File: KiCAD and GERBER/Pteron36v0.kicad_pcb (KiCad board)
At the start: 2 copper layers, 140.1 x 108.1 mm, 56 parts, among them J1 AudioJack4, J2 AudioJack4, J3 Conn_01x04, SW10 SW_PUSH, SW12 SW_PUSH, SW13 SW_PUSH, SW14 SW_PUSH, SW15 SW_PUSH, SW17 SW_PUSH, SW18 SW_PUSH, SW19 SW_PUSH, SW20 SW_PUSH, SW22 SW_PUSH, SW23 SW_PUSH, SW24 SW_PUSH, SW26 SW_PUSH, SW27 SW_PUSH, SW28 SW_PUSH, SW7 SW_PUSH, SW8 SW_PUSH, SW9 SW_PUSH, U1 ProMicro

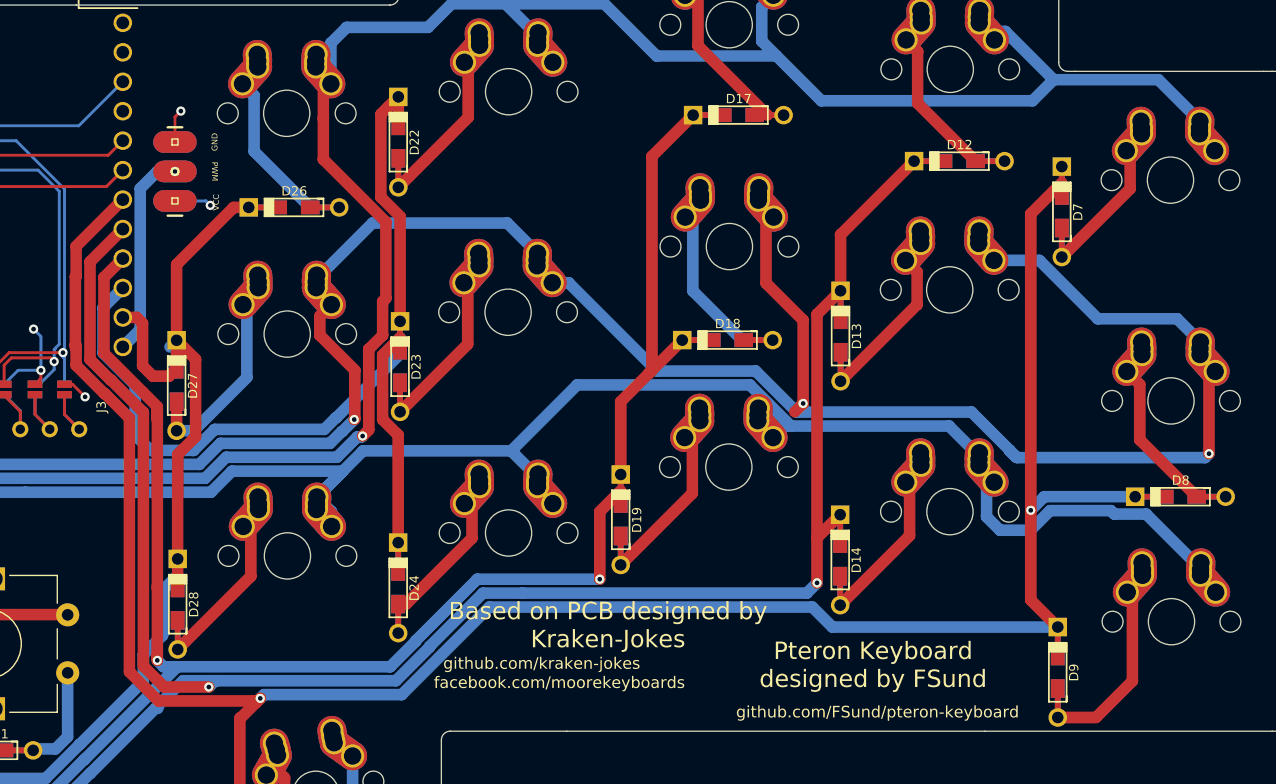
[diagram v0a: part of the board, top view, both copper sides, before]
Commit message: updated pcb
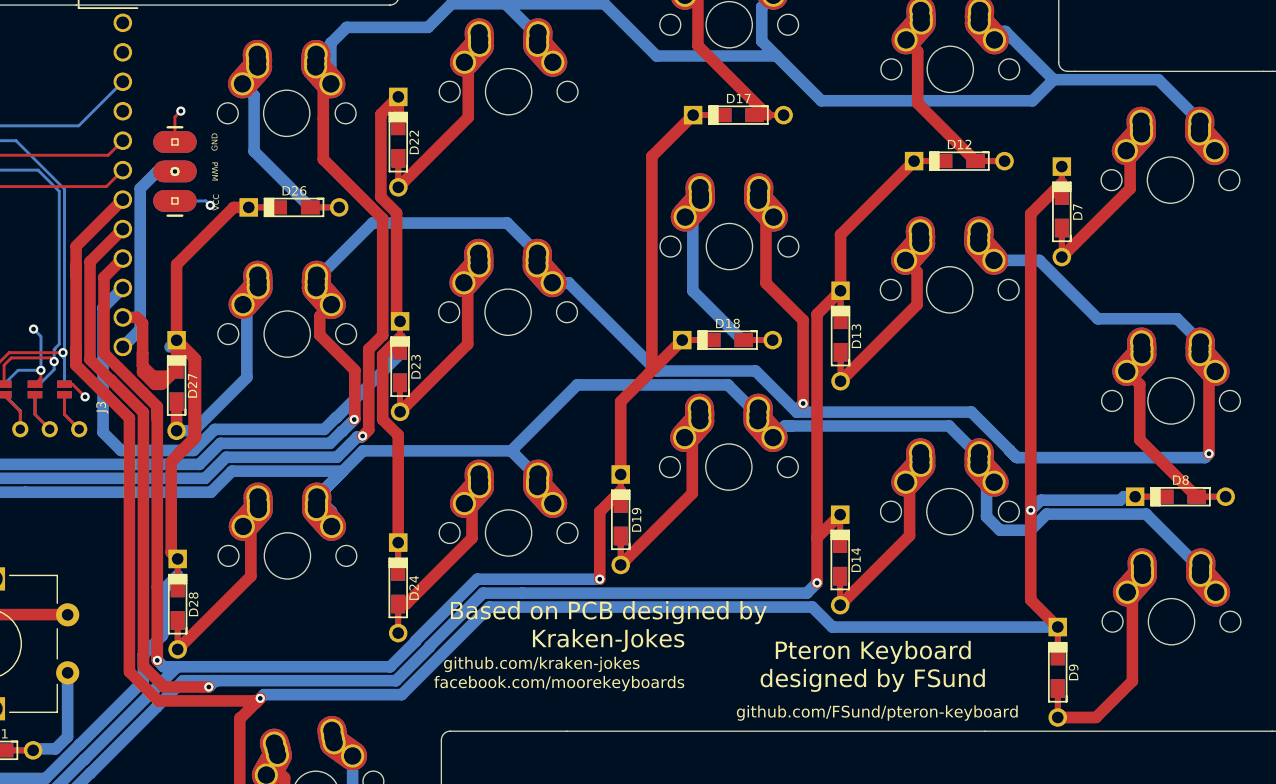
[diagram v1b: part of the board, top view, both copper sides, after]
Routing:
- net /Col5: track 80.6 -> 96.3 mm
- net /Row3: track 151.3 -> 147.8 mm
- net /Col1: track 201.2 -> 203.4 mm
- net /Col4: track 83.7 -> 85.2 mm
- net /Row2: track 201.5 -> 200.5 mm
